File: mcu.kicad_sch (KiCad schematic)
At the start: 5 parts, among them IC4 STM32G0B1CBT6N

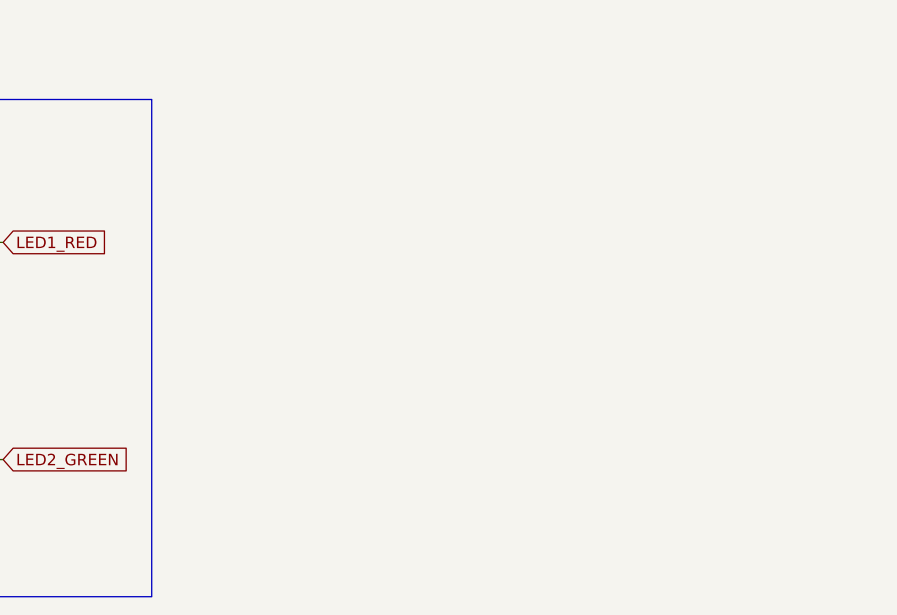
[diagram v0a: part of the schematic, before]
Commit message: First Layout Try
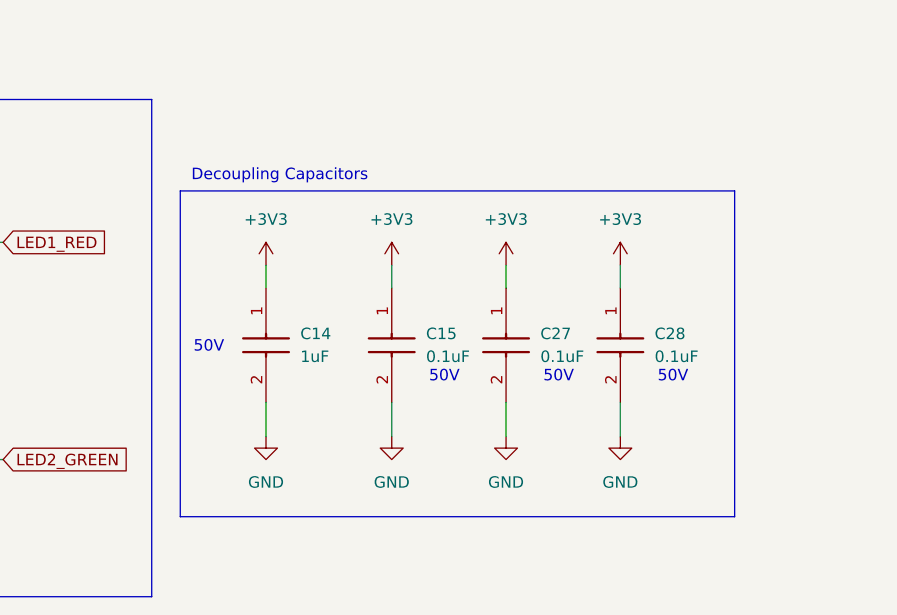
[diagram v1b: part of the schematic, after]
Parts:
- added C14: 1uF, C2012X7R1H105K125AB:CAPC2012X145N, symbol C2012X7R1H105K125AB:C2012X7R1H105K125AB
- added C15, C27, C28: 0.1uF, CC0603KRX7R9BB104:CAPC1608X90N, symbol CC0603KRX7R9BB104:CC0603KRX7R9BB104
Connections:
- net +3V3: now also C14.1, C15.1, C27.1, C28.1
- net GND: now also C14.2, C15.2, C27.2, C28.2
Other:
- note added: "50V"
- note added: "Decoupling Capacitors"

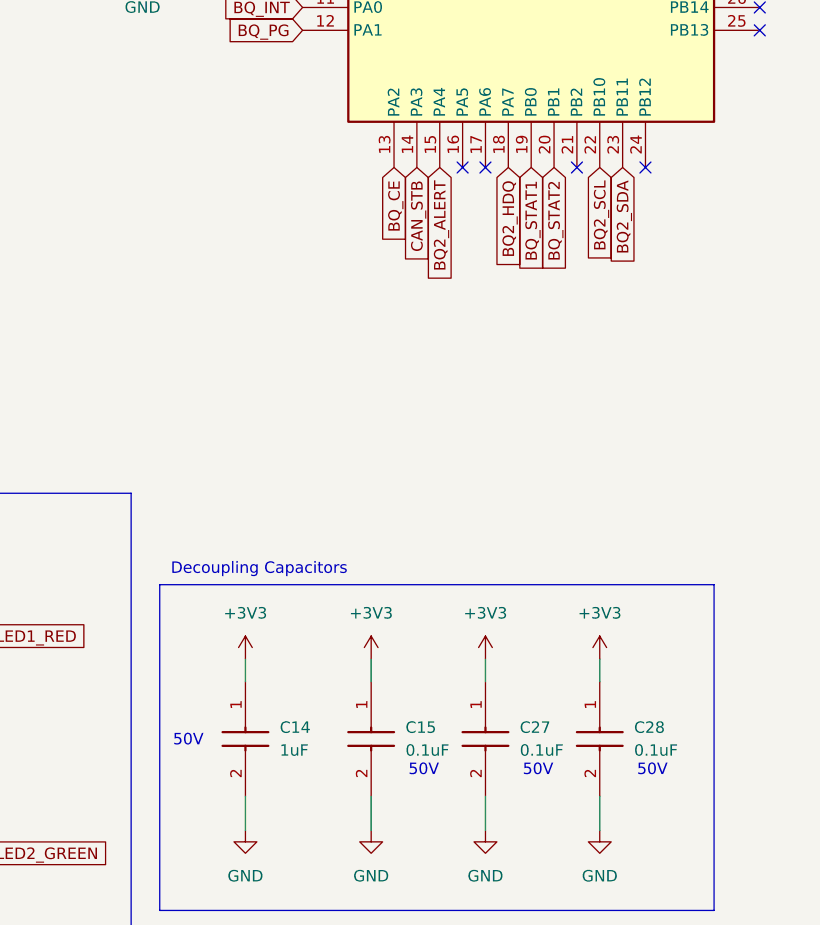
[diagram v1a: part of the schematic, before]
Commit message: First Changes
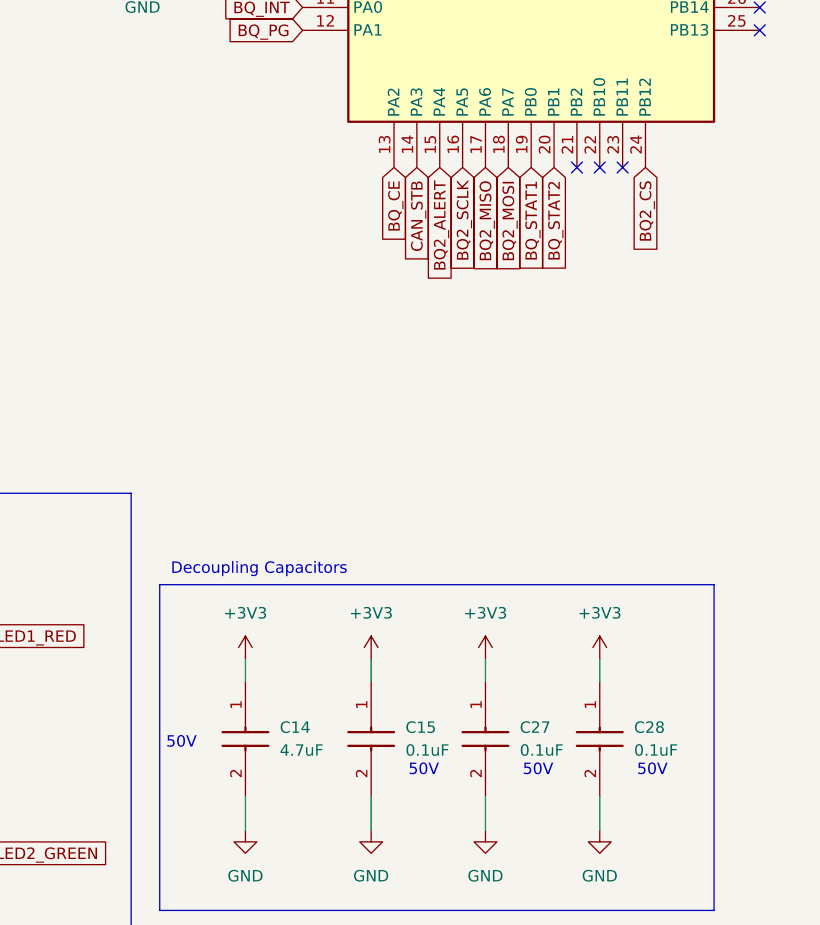
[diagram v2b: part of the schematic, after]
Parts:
- removed C14: 1uF, C2012X7R1H105K125AB:CAPC2012X145N, symbol C2012X7R1H105K125AB:C2012X7R1H105K125AB
- added C14: 4.7uF, UMJ325AB7475KMHP:CAPC3225X280N, symbol UMJ325AB7475KMHP:UMJ325AB7475KMHP
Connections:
- net +3V3: now also C14.1
- net GND: now also C14.2
- net BQ2_SCLK: now reaches IC4.16 (PA5)
- net BQ2_MISO: now reaches IC4.17 (PA6)
- net BQ2_CS: now reaches IC4.24 (PB12)
- net BQ2_HDQ renamed BQ2_MOSI
- net BQ2_SCL: no longer names the net of IC4.22 (PB10)
- net BQ2_SDA: no longer names the net of IC4.23 (PB11)
- no-connect marks 23 -> 22
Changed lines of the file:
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@@
 	(text "50V"
 		(exclude_from_sim no)
-		(at 104.14 161.544 0)
+		(at 103.378 161.798 0)
 		(effects
 			(font
@@
 	)
 	(no_connect
-		(at 137.16 97.79)
+		(at 152.4 97.79)
 	)
 	(no_connect
@@
 	)
 	(no_connect
-		(at 134.62 97.79)
-	)
-	(no_connect
 		(at 149.86 39.37)
-	)
-	(no_connect
-		(at 154.94 97.79)
 	)
 	(no_connect
@@
 	(no_connect
 		(at 167.64 82.55)
+	)
+	(no_connect
+		(at 149.86 97.79)
 	)
 	(no_connect
@@
 		)
 	)
-	(global_label "BQ2_HDQ"
+	(global_label "BQ2_MOSI"
 		(shape input)
 		(at 139.7 97.79 270)
@@
 		)
 		(property "Intersheetrefs" "${INTERSHEET_REFS}"
-			(at 139.7 109.4838 90)
+			(at 139.7 110.149 90)
 			(effects
 				(font
@@
 		)
 	)
+	(global_label "BQ2_CS"
+		(shape input)
+		(at 154.94 97.79 270)
+		(fields_autoplaced yes)
+		(effects
+			(font
+				(size 1.27 1.27)
+			)
+			(justify right)
+		)
+		(property "Intersheetrefs" "${INTERSHEET_REFS}"
+			(at 154.94 108.0323 90)
+			(effects
+				(font
+					(size 1.27 1.27)
+				)
+				(justify right)
+				(hide yes)
+			)
+		)
+	)
 	(global_label "LED1_RED"
 		(shape input)
@@
 		)
 	)
+	(global_label "BQ2_SCLK"
+		(shape input)
+		(at 134.62 97.79 270)
+		(fields_autoplaced yes)
+		(effects
+			(font
+				(size 1.27 1.27)
+			)
+			(justify right)
+		)
+		(property "Intersheetrefs" "${INTERSHEET_REFS}"
+			(at 134.62 110.3304 90)
+			(effects
+				(font
+					(size 1.27 1.27)
+				)
+				(justify right)
+				(hide yes)
+			)
+		)
+	)
 	(global_label "SWCLK"
 		(shape input)
@@
 		)
 	)
-	(global_label "BQ2_SDA"
-		(shape input)
-		(at 152.4 97.79 270)
-		(fields_autoplaced yes)
-		(effects
-			(font
-				(size 1.27 1.27)
-			)
-			(justify right)
-		)
-		(property "Intersheetrefs" "${INTERSHEET_REFS}"
-			(at 152.4 109.1209 90)
-			(effects
-				(font
-					(size 1.27 1.27)
-				)
-				(justify right)
-				(hide yes)
-			)
-		)
-	)
 	(global_label "BQ_STAT2"
 		(shape input)
@@
 		)
 	)
-	(global_label "BQ2_SCL"
-		(shape input)
-		(at 149.86 97.79 270)
-		(fields_autoplaced yes)
-		(effects
-			(font
-				(size 1.27 1.27)
-			)
-			(justify right)
-		)
-		(property "Intersheetrefs" "${INTERSHEET_REFS}"
-			(at 149.86 109.0604 90)
-			(effects
-				(font
-					(size 1.27 1.27)
-				)
-				(justify right)
-				(hide yes)
-			)
-		)
-	)
 	(global_label "BQ_INT"
 		(shape input)
@@
 		(property "Intersheetrefs" "${INTERSHEET_REFS}"
 			(at 107.3838 80.01 0)
+			(effects
+				(font
+					(size 1.27 1.27)
+				)
+				(justify right)
+				(hide yes)
+			)
+		)
+	)
+	(global_label "BQ2_MISO"
+		(shape input)
+		(at 137.16 97.79 270)
+		(fields_autoplaced yes)
+		(effects
+			(font
+				(size 1.27 1.27)
+			)
+			(justify right)
+		)
+		(property "Intersheetrefs" "${INTERSHEET_REFS}"
+			(at 137.16 110.149 90)
 			(effects
 				(font
@@
 	)
 	(symbol
-		(lib_id "C2012X7R1H105K125AB:C2012X7R1H105K125AB")
-		(at 110.49 154.94 270)
-		(unit 1)
-		(exclude_from_sim no)
-		(in_bom yes)
-		(on_board yes)
-		(dnp no)
-		(fields_autoplaced yes)
-		(property "Reference" "C14"
-			(at 114.3 160.0199 90)
-			(effects
-				(font
-					(size 1.27 1.27)
-				)
-				(justify left)
-			)
-		)
-		(property "Value" "1uF"
-			(at 114.3 162.5599 90)
-			(effects
-				(font
-					(size 1.27 1.27)
-				)
-				(justify left)
-			)
-		)
-		(property "Footprint" "C2012X7R1H105K125AB:CAPC2012X145N"
-			(at 14.3 163.83 0)
-			(effects
-				(font
-					(size 1.27 1.27)
-				)
-				(justify left top)
-				(hide yes)
-			)
-		)
-		(property "Datasheet" "https://product.tdk.com/info/en/catalog/datasheets/mlcc_commercial_midvoltage_en.pdf"
-			(at -85.7 163.83 0)
-			(effects
-				(font
-					(size 1.27 1.27)
-				)
-				(justify left top)
-				(hide yes)
-			)
-		)
-		(property "Description" "MULTILAYER CERAMIC CHIP CAPACITORS, 2012, Commercial grade, general (Up to 75V)"
-			(at 110.49 154.94 0)
-			(effects
-				(font
-					(size 1.27 1.27)
-				)
-				(hide yes)
-			)
-		)
-		(property "Height" "1.45"
-			(at -285.7 163.83 0)
-			(effects
-				(font
-					(size 1.27 1.27)
-				)
-				(justify left top)
-				(hide yes)
-			)
-		)
-		(property "Mouser Part Number" "810-C2012X7R1H105K"
-			(at -385.7 163.83 0)
-			(effects
-				(font
-					(size 1.27 1.27)
-				)
-				(justify left top)
-				(hide yes)
-			)
-		)
-		(property "Mouser Price/Stock" "https://www.mouser.co.uk/ProductDetail/TDK/C2012X7R1H105K125AB?qs=NRhsANhppD9AlYlb8kBg7Q%3D%3D"
-			(at -485.7 163.83 0)
-			(effects
-				(font
-					(size 1.27 1.27)
-				)
-				(justify left top)
-				(hide yes)
-			)
-		)
-		(property "Manufacturer_Name" "TDK"
-			(at -585.7 163.83 0)
-			(effects
-				(font
-					(size 1.27 1.27)
-				)
-				(justify left top)
-				(hide yes)
-			)
-		)
-		(property "Manufacturer_Part_Number" "C2012X7R1H105K125AB"
-			(at -685.7 163.83 0)
-			(effects
-				(font
-					(size 1.27 1.27)
-				)
-				(justify left top)
-				(hide yes)
-			)
-		)
-		(pin "1"
-		)
-		(pin "2"
-		)
-		(instances
-			(project "Lithium_Board"
-				(path "/a208389b-7ee7-48d8-95f2-b3e129849547/160492a7-828d-4540-9766-a6c613c08096"
-					(reference "C14")
-					(unit 1)
-				)
-			)
-		)
-	)
-	(symbol
 		(lib_id "power:+3V3")
 		(at 124.46 152.4 0)
@@
 					(unit 1)
 				)
+			)
+		)
+	)
+	(symbol
+		(lib_id "UMJ325AB7475KMHP:UMJ325AB7475KMHP")
+		(at 110.49 154.94 270)
+		(unit 1)
+		(exclude_from_sim no)
+		(in_bom yes)
+		(on_board yes)
+		(dnp no)
+		(fields_autoplaced yes)
+		(property "Reference" "C14"
+			(at 114.3 160.0199 90)
+			(effects
+				(font
+					(size 1.27 1.27)
+				)
+				(justify left)
+			)
+		)
+		(property "Value" "4.7uF"
+			(at 114.3 162.5599 90)
+			(effects
+				(font
+					(size 1.27 1.27)
+				)
+				(justify left)
+			)
+		)
+		(property "Footprint" "UMJ325AB7475KMHP:CAPC3225X280N"
+			(at 14.3 163.83 0)
+			(effects
+				(font
+					(size 1.27 1.27)
+				)
+				(justify left top)
+				(hide yes)
+			)
+		)
+		(property "Datasheet" "https://ds.yuden.co.jp/TYCOMPAS/or/specSheet?pn=MCJCU32MAB7475KPPA01"
+			(at -85.7 163.83 0)
+			(effects
+				(font
+					(size 1.27 1.27)
+				)
+				(justify left top)
+				(hide yes)
+			)
+		)
+		(property "Description" "4.7 F +/-10% 50V Ceramic Capacitor X7R 1210 (3225 Metric)"
+			(at 110.49 154.94 0)
+			(effects
+				(font
+					(size 1.27 1.27)
+				)
+				(hide yes)
+			)
+		)
+		(property "Height" "2.8"
+			(at -285.7 163.83 0)
+			(effects
+				(font
+					(size 1.27 1.27)
+				)
+				(justify left top)
+				(hide yes)
+			)
+		)
+		(property "Mouser Part Number" "963-UMJ325AB7475KMHP"
+			(at -385.7 163.83 0)
+			(effects
+				(font
+					(size 1.27 1.27)
+				)
+				(justify left top)
+				(hide yes)
+			)
+		)
+		(property "Mouser Price/Stock" "https://www.mouser.co.uk/ProductDetail/TAIYO-YUDEN/UMJ325AB7475KMHP?qs=sBf%2Fb4nBSlehnKp%252BnIaW0Q%3D%3D"
+			(at -485.7 163.83 0)
+			(effects
+				(font
+					(size 1.27 1.27)
+				)
+				(justify left top)
+				(hide yes)
+			)
+		)
+		(property "Manufacturer_Name" "TAIYO YUDEN"
+			(at -585.7 163.83 0)
+			(effects
+				(font
+					(size 1.27 1.27)
+				)
+				(justify left top)
+				(hide yes)
+			)
+		)
+		(property "Manufacturer_Part_Number" "UMJ325AB7475KMHP"
+			(at -685.7 163.83 0)
+			(effects
+				(font
+					(size 1.27 1.27)
+				)
+				(justify left top)
+				(hide yes)
+			)
+		)
+		(pin "2"
+		)
+		(pin "1"
+		)
+		(instances
+			(project "Lithium_Board"
+				(path "/a208389b-7ee7-48d8-95f2-b3e129849547/160492a7-828d-4540-9766-a6c613c08096"
+					(reference "C14")
+					(unit 1)
+				)
